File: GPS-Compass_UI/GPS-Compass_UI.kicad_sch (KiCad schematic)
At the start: 28 parts, among them J3 FFC2B28-12-G, SW1 SPDT, SW2 EXT, SW3 RESET, SW4 RESET, SW5 EXT, SW6 EXT, SW7 EXT

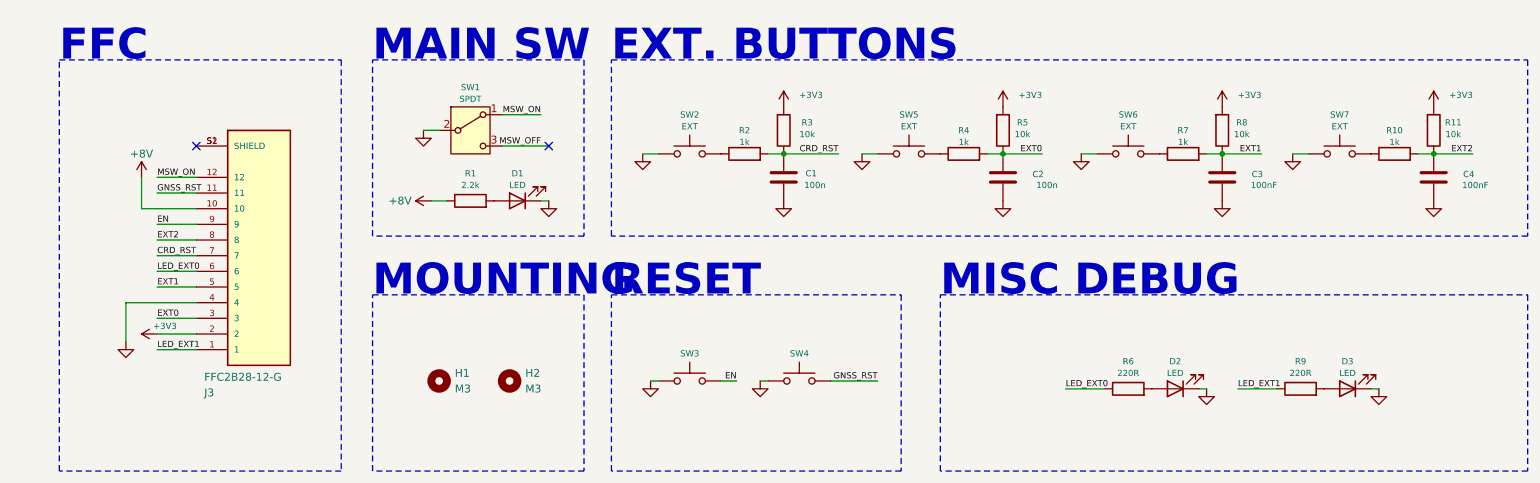
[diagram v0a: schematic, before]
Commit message: UI changes
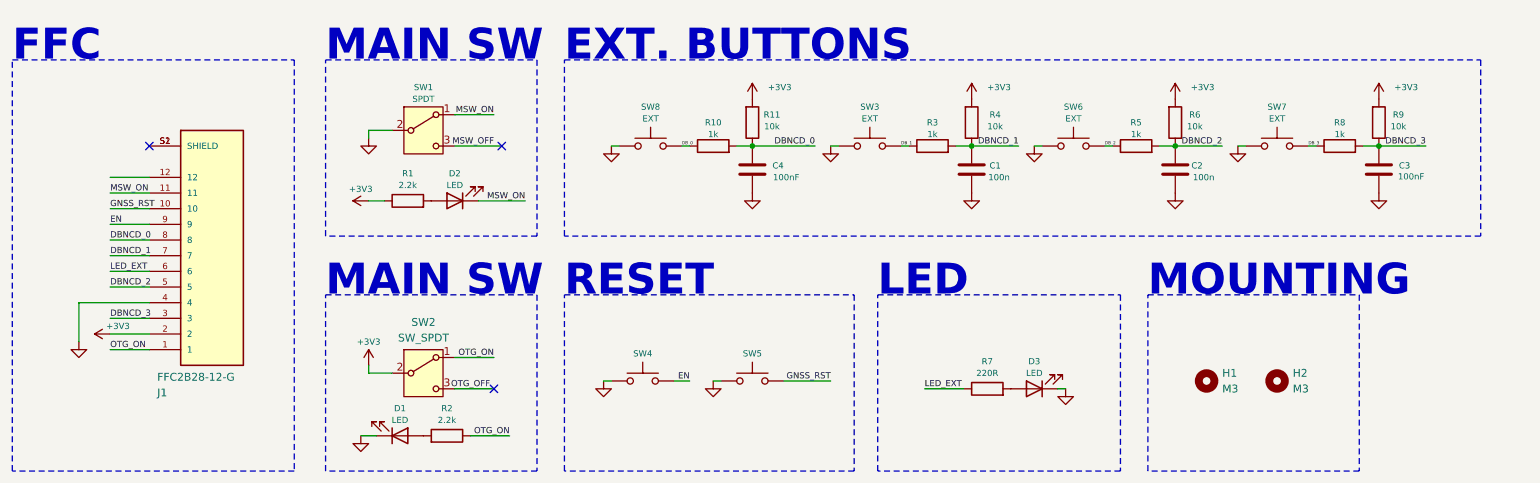
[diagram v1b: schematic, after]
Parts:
- removed D3: LED, Connector_Wire:SolderWire-0.1sqmm_1x02_P3.6mm_D0.4mm_OD1mm_Relief, symbol Device:LED
- removed R9: 220R, Resistor_SMD:R_0805_2012Metric, symbol Device:R
- added D1: LED, Connector_Wire:SolderWire-0.1sqmm_1x02_P3.6mm_D0.4mm_OD1mm_Relief, symbol Device:LED
- added R2: 2.2k, Resistor_SMD:R_0805_2012Metric, symbol Device:R
- added SW2: SW_SPDT, Connector_Wire:SolderWire-0.1sqmm_1x02_P3.6mm_D0.4mm_OD1mm_Relief, symbol Switch:SW_SPDT
- renumbered D1 to D2, D2 to D3, J3 to J1, R2 to R3, R3 to R4, R4 to R5, R5 to R6, R6 to R7, R7 to R8, R8 to R9, SW2 to SW3, SW3 to SW4, SW4 to SW5, SW5 to SW6, SW6 to SW7, SW7 to SW8
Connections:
- net +3V3: now also R1.1, SW2.2 (B)
- net GND: now also D1.1 (K); no longer D2.1 (K)
- net GNSS_RST: now also J1.10; no longer J1.11
- net MSW_ON: now also D2.1 (K), J1.11; no longer J1.12
- net DB_1: now reaches R3.1, SW3.2
- net DB_3: now reaches R8.1, SW7.2
- net DB_0: now reaches R10.1, SW8.2
- net DB_2: now reaches R5.1, SW6.2
- removed net +8V: J1.10, R1.1
- net CRD_RST renamed DBNCD_1
- net EXT0 renamed DBNCD_2
- net DBNCD_2: now also J1.5; no longer J1.3
- net EXT1 renamed DBNCD_3
- net DBNCD_3: now also J1.3; no longer J1.5
- net EXT2 renamed DBNCD_0
- net LED_EXT0 renamed LED_EXT
- net LED_EXT1 renamed OTG_ON
- net OTG_ON: now also R2.1, SW2.1 (A)
- new net: D1.2 (A), R2.2
- new net OTG_OFF: SW2.3 (C)
- no-connect marks 2 -> 3
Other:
- note added: "LED"
- note removed: "MISC DEBUG"
- moved on the sheet: C1, C2, C3, C4, D2, D3, H1, H2, J1, R1, R10, R11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
